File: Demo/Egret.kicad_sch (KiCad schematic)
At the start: 28 parts, among them J1 Micro_SD_Card, J2 2388749-1, Q1 S8050, Q2 S8050, U1 MPU6050, U2 LP2992IM5-3.3, U3 WS2812B-B, U4 CP2102N-A01-GQFN28, U5 ESP32-PICO-D4, U6 AN2051

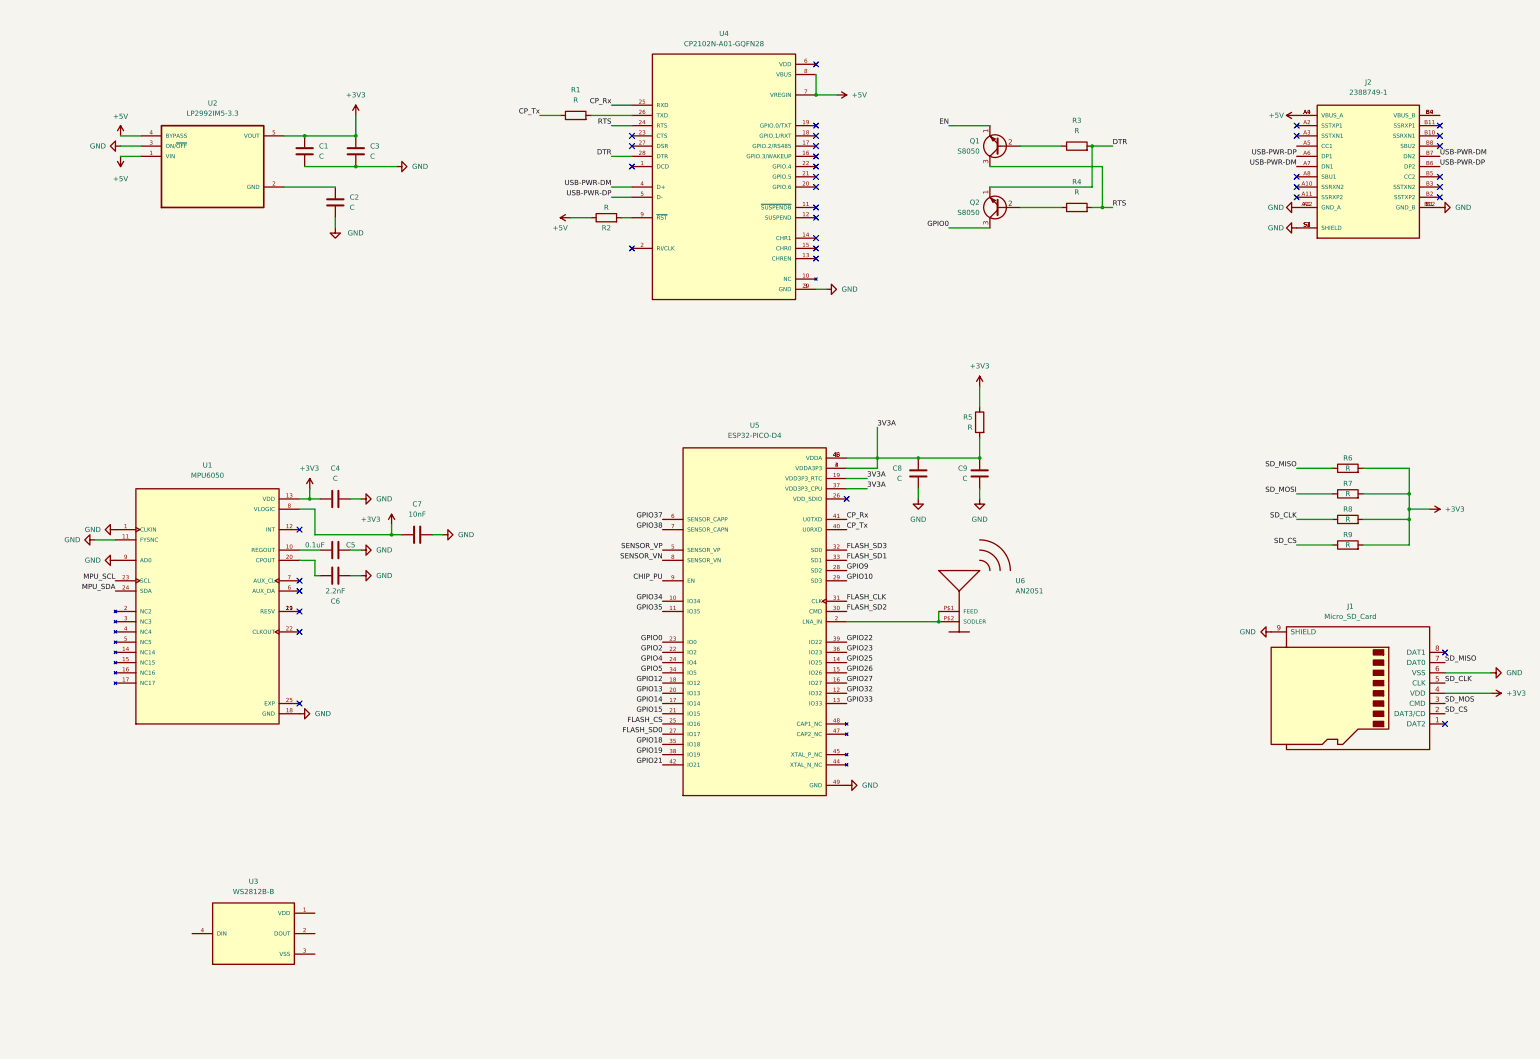
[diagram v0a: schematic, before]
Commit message: update
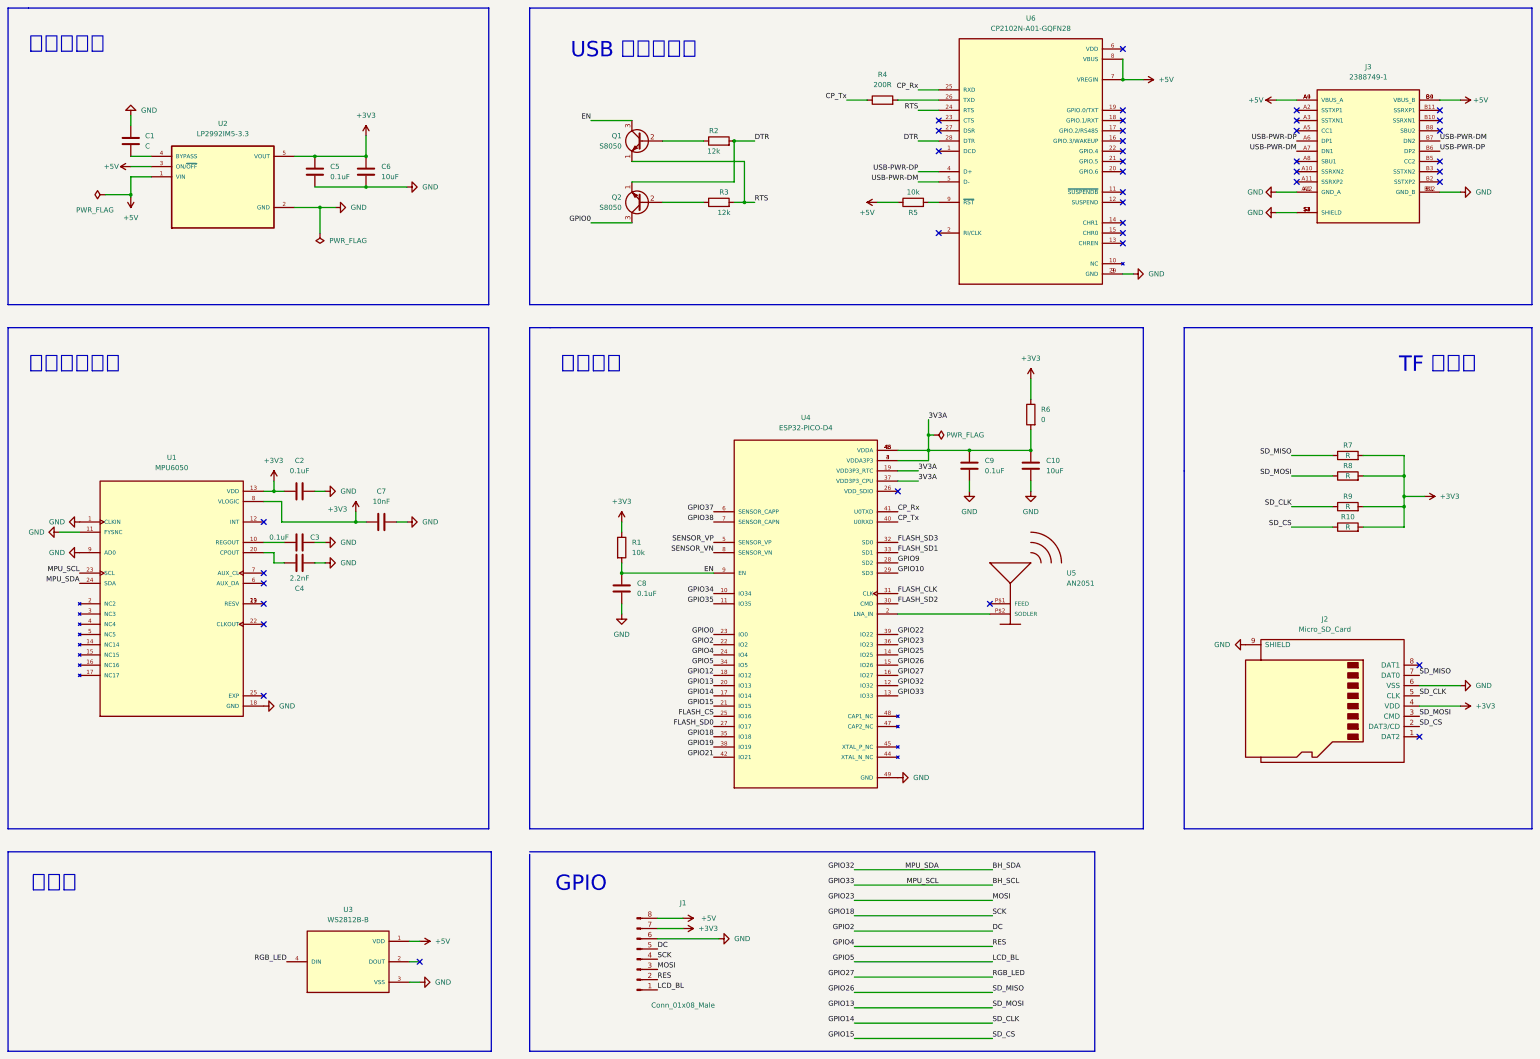
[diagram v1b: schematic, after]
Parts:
- added C8: 0.1uF, symbol Device:C
- added J1: Conn_01x08_Male, symbol Connector:Conn_01x08_Male
- added R1: 10k, symbol Device:R
- C10: renamed from C9; value C -> 10uF
- C2: renamed from C4; value C -> 0.1uF
- C5: renamed from C1; value C -> 0.1uF
- C6: renamed from C3; value C -> 10uF
- C9: renamed from C8; value C -> 0.1uF
- R2: renamed from R3; value R -> 12k
- R3: renamed from R4; value R -> 12k
- R4: renamed from R1; value R -> 200R
- R5: renamed from R2; value R -> 10k
- R6: renamed from R5; value R -> 0
- renumbered C2 to C1, C5 to C3, C6 to C4, J1 to J2, J2 to J3, R9 to R10, R6 to R7, R7 to R8, R8 to R9, U5 to U4, U6 to U5, U4 to U6
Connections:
- net CHIP_PU is gone; now on net EN: U4.9 (EN)
- net MPU_SCL is gone; now on net BH_SCL: U1.23 (SCL)
- net MPU_SDA is gone; now on net BH_SDA: U1.24 (SDA)
- net SD_CLK is gone; now on net GPIO14: J2.5 (CLK), R9.1
- net SD_CS is gone; now on net GPIO15: J2.2 (DAT3/CD), R10.1
- net SD_MISO is gone; now on net GPIO26: J2.7 (DAT0), R7.1
- net SD_MOS is gone; now on net GPIO13: J2.3 (CMD)
- net SD_MOSI is gone; now on net GPIO13: R8.1
- net +3V3: now also J1.7 (Pin_7), R1.1
- net +5V: now also J3.B4 (VBUS_B), J3.B9 (VBUS_B), U2.3 (ON/~{OFF}), U3.1 (VDD), J1.8 (Pin_8); no longer U2.4 (BYPASS)
- net EN: now also Q1.3 (C), C8.1, R1.2; no longer Q1.1 (E)
- net GND: now also C1.2, U2.2 (GND), U3.3 (VSS), C8.2, J1.6 (Pin_6); no longer C1.1, U2.3 (ON/~{OFF})
- net GPIO18: now also J1.4 (Pin_4)
- net GPIO23: now also J1.3 (Pin_3)
- net GPIO27: now also U3.4 (DIN)
- net GPIO4: now also J1.2 (Pin_2)
- net GPIO5: now also J1.1 (Pin_1)
- net RTS: now also Q1.1 (E); no longer Q1.3 (C)
- net USB-PWR-DM: now also U6.5 (D-); no longer U6.4 (D+)
- net USB-PWR-DP: now also U6.4 (D+); no longer U6.5 (D-)
- net at U4.2 (LNA_IN), U5.P$2 (SODLER): no longer U5.P$1 (FEED)
- net GPIO2 renamed DC
- net DC: now also J1.5 (Pin_5)
- net GPIO32 renamed BH_SDA
- net GPIO33 renamed BH_SCL
- new net: C1.1, U2.4 (BYPASS)
- no-connect marks 37 -> 40
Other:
- note added: "GPIO"
- note added: "TF 存储卡"
- note added: "USB 转串口芯片"
- note added: "加速度传感器"
- note added: "微控制器"
- note added: "扩展板"
- note added: "线性稳压器"
- moved on the sheet: C1, C10, C2, C3, C4, C5, C6, C7, C9, J2, J3, Q1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
